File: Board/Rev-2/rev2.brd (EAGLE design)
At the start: 148.6 x 63.2 mm, 56 parts, among them IC1 74HC595N, T1 2N3904, T2 2N3904, T3 2N3904, T4 2N3904, T5 2N3904, T6 2N3904, T7 2N3904, T8 2N3904

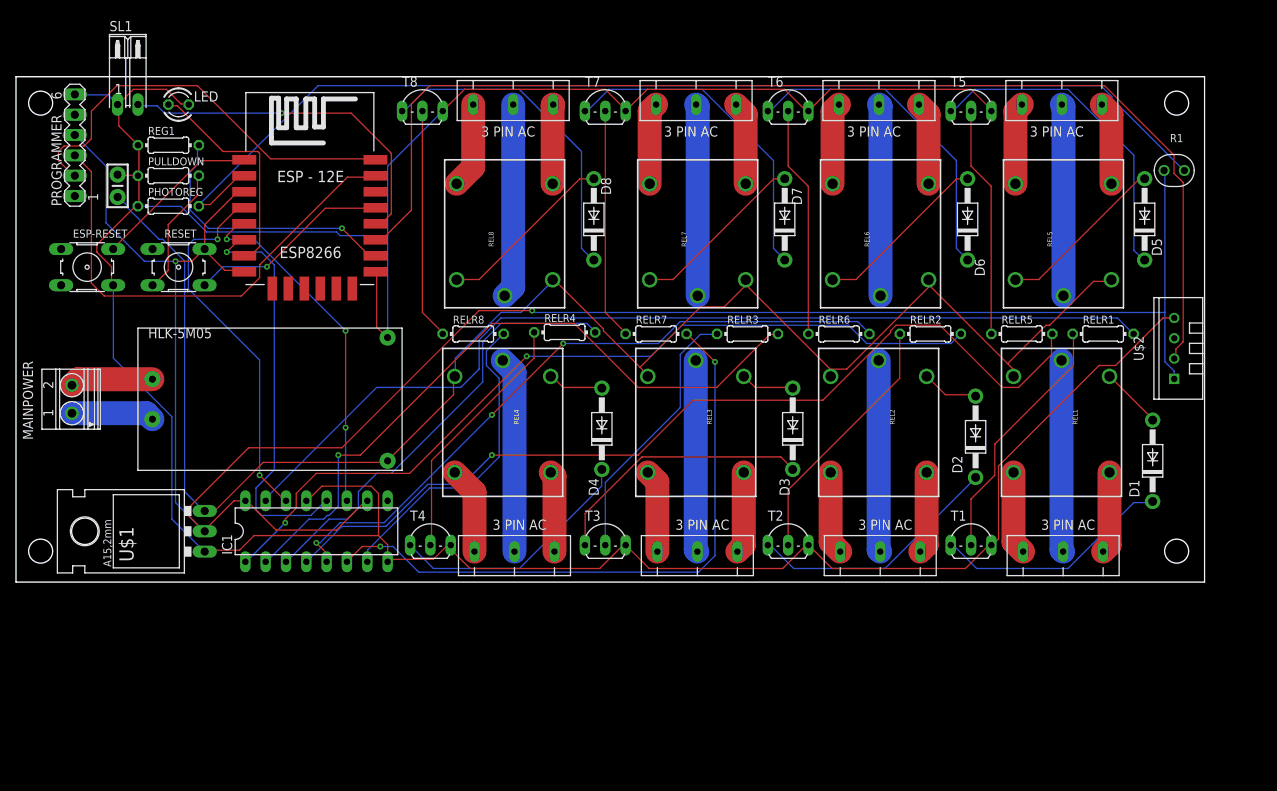
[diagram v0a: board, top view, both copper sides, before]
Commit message: Board Generated
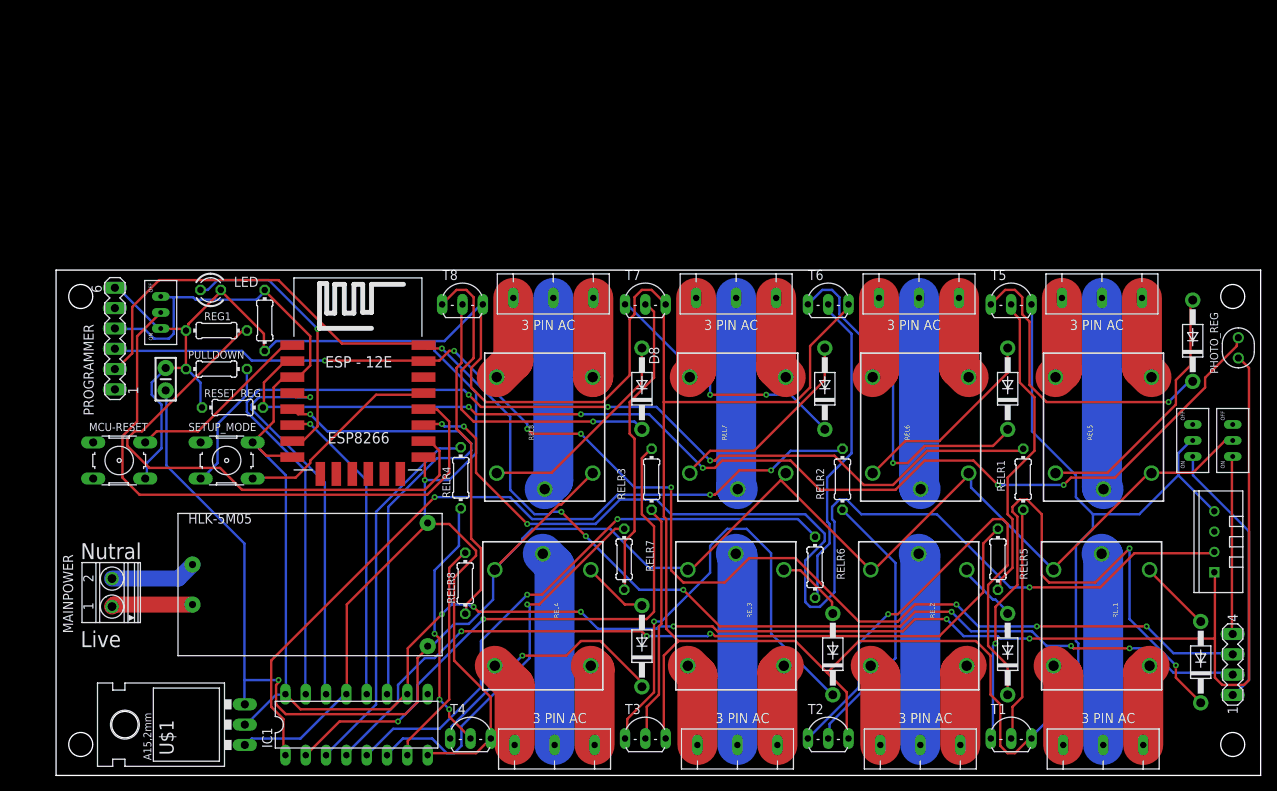
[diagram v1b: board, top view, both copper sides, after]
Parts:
- removed ESP-RESET, RESET: tackswitch, buttons:B3F-10XX
- removed PHOTOREG: 1kohm, resistor:0204/7
- removed R1: PHOTOCELLONB, LDR:ON_BOARD
- removed SL1: Flash, con-amp-quick:02PA
- added FLASH, GND_SWITCH, VCC_SWITCH: TOGGLE_SWITCH, Toggle Switch:TOGGLE_SWITCH
- added MCU-RESET, SETUP_MODE: tackswitch, buttons:B3F-10XX
- added PHOTO_REG: PHOTOCELLONB, LDR:ON_BOARD
- added PULLUP: 10kohm, resistor:0204/7
- added RESET_REG: 1kohm, resistor:0204/7
- added SV1: (no value), con-lstb:MA04-1
- moved RELR8 31.2 mm to (51.1, 24.0), turned to 90 degrees
- moved RELR6 29.3 mm to (94.8, 26.0), turned to 90 degrees
- moved D3 28.6 mm to (97.0, 15.1)
- moved RELR7 28.5 mm to (70.9, 27.0), turned to 90 degrees
- moved RELR5 28.3 mm to (117.7, 27.0), turned to 90 degrees
- moved D4 27.6 mm to (73.2, 16.1)
- moved D2 27.5 mm to (118.9, 15.1)
- moved D1 25.9 mm to (143.0, 14.1)
- moved PULLDOWN 24.9 mm to (20.0, 50.8)
- moved C1 24.9 mm to (13.6, 49.5)
- moved T5 24.7 mm to (119.3, 60.1)
- moved T6 24.7 mm to (96.4, 60.1)
- moved T8 24.7 mm to (50.7, 60.1)
- moved U$2 24.7 mm to (144.7, 29.2)
- moved CON-REL-1 24.7 mm to (135.8, 3.77)
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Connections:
- new net N$55: GND_SWITCH.ON, SV1.1
- new net N$56: SV1.4, VCC_SWITCH.ON
- net 3.5V: now also FLASH.OFF, PHOTO_REG.1, PULLUP.2, SETUP_MODE.2; no longer R1.1, RESET.2
- net ADC: now also PHOTO_REG.2, RESET_REG.2; no longer PHOTOREG.2, R1.2
- net GND: now also FLASH.ON, GND_SWITCH.IN, MCU-RESET.4, PULLUP.1, RESET_REG.1; no longer ESP-RESET.4, PHOTOREG.1, SL1.1
- net N$26: now also SETUP_MODE.4; no longer RESET.4
- net N$28: now also FLASH.IN; no longer SL1.2
- net N$29: now also SETUP_MODE.3; no longer RESET.3
- net N$31: now also MCU-RESET.2; no longer ESP-RESET.2
- net RX: now also SV1.2
- net TX: now also SV1.3
- net VCC: now also VCC_SWITCH.IN
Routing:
- net RX: track 52.8 -> 175.5 mm, vias 0 -> 7
- net TX: track 60.3 -> 167.4 mm, vias 0 -> 8
- net GND: track 399.1 -> 492.8 mm, vias 0 -> 1
- net N$47: track 30.0 -> 79.1 mm, vias 0 -> 3
- net N$27: track 34.1 -> 69.1 mm, vias 1 -> 0
- net N$55: track 0.00 -> 33.6 mm
- net N$28: track 44.2 -> 75.7 mm, vias 1 -> 0
- net N$48: track 32.0 -> 63.2 mm, vias 0 -> 1
- net RELAY7: track 78.2 -> 48.7 mm, vias 2 -> 1
- net VCC: track 206.3 -> 234.3 mm, vias 0 -> 1
- net N$49: track 33.5 -> 59.7 mm, vias 0 -> 1
- net RELAY1: track 121.2 -> 144.6 mm, vias 0 -> 3
- net N$56: track 0.00 -> 22.3 mm
- net 3.5V: track 266.5 -> 285.4 mm, vias 2 -> 6
- net SHCP: track 44.3 -> 61.8 mm, vias 3 -> 1
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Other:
- board size 148.6 x 63.2 mm -> 150.6 x 63.2 mm
- board text added: "Live"
- board text added: "Nutral"
